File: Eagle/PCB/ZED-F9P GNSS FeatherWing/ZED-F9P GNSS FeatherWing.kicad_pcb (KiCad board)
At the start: 2 copper layers, 50.8 x 22.9 mm, 43 parts, among them CON1 MICROBUILDER_USBFCI_10103594_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, J1 Coupler_v2_Coupler_v2-rescue_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, Q1 DMG2305, U1 ZED-F9P_ZED-F9P, U2 SPX3819-3.3, X1 SMA-142-0711-821/826

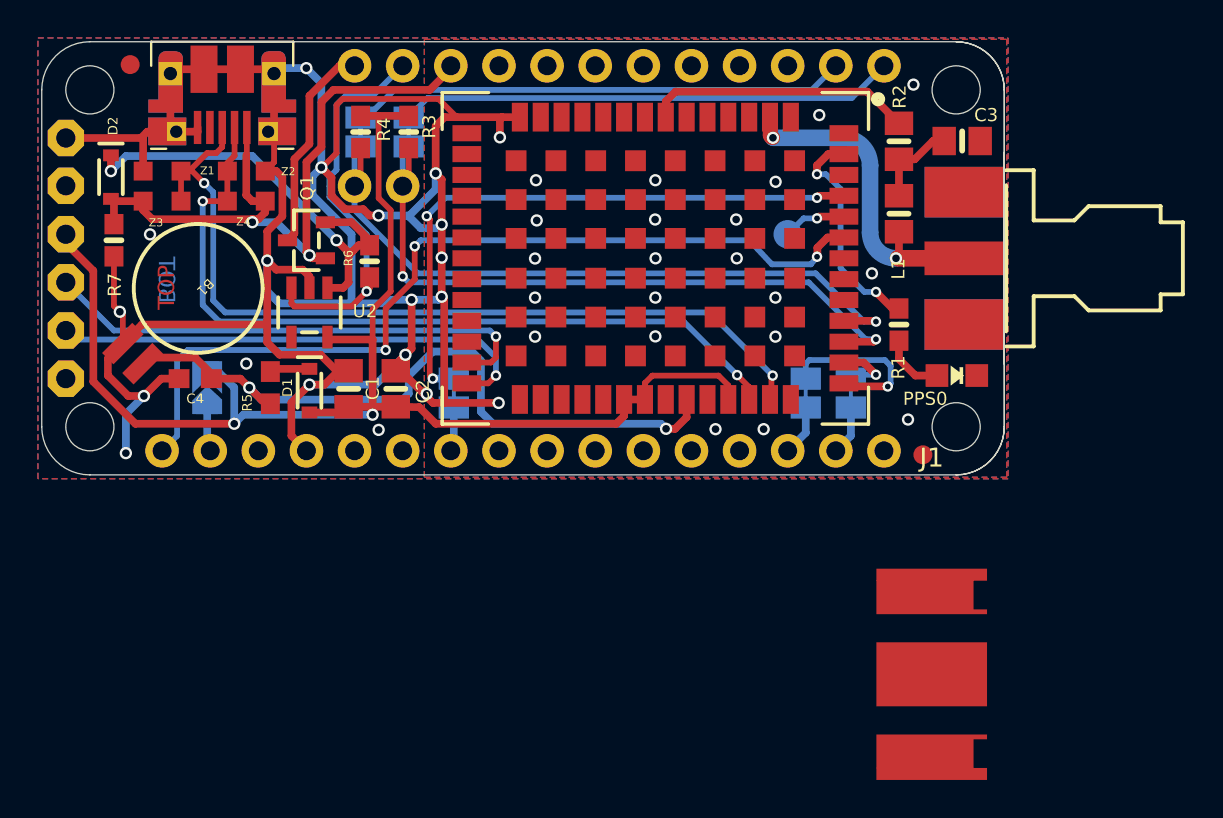
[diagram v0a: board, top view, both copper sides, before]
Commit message: V2 Release
Released to fab.
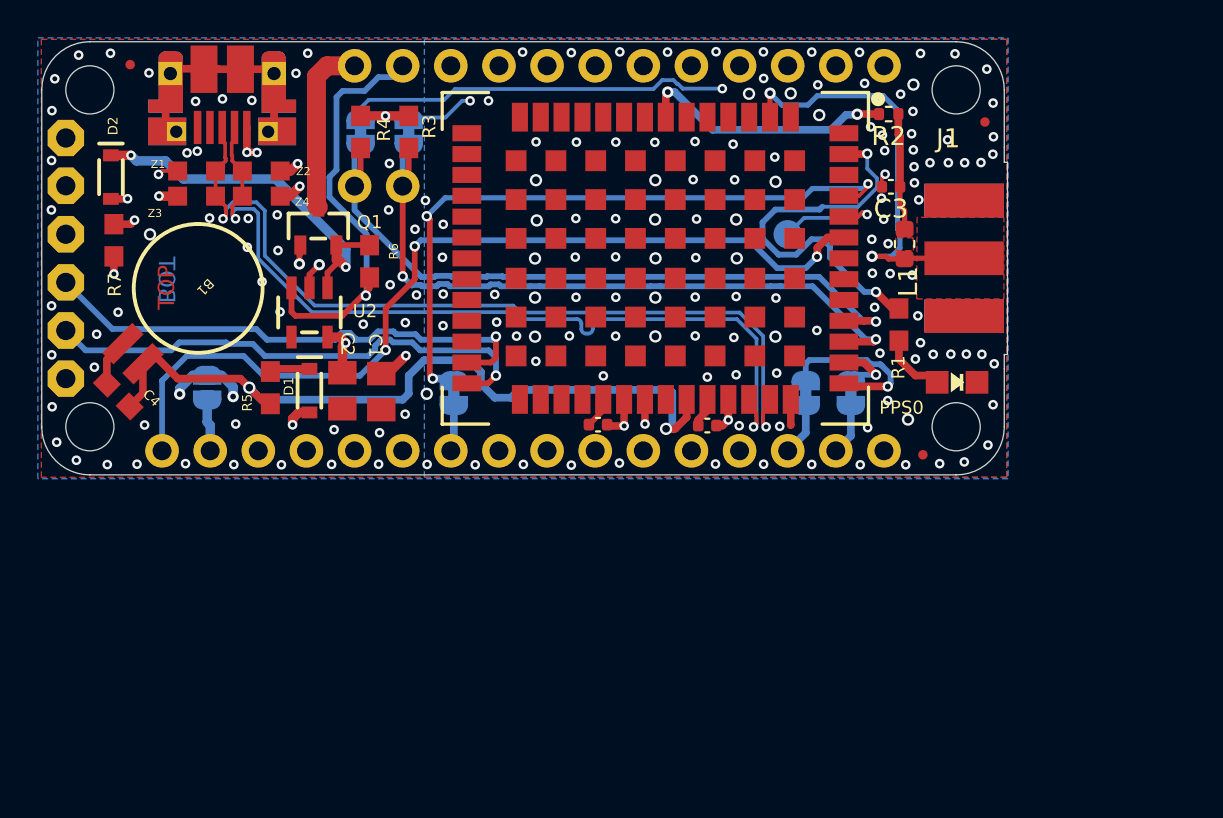
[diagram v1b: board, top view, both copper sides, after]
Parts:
- removed X1: SMA-142-0711-821/826, ZED-F9P GNSS FeatherWing:J502-ND-142-0711-821_826_133
- added C5: C_Small_US, Capacitor_SMD:C_0402_1005Metric, F.Cu at (158.2, 113.8)
- added C6: C_Small_US, Capacitor_SMD:C_0402_1005Metric, F.Cu at (152.5, 113.8)
- added FID3: FIDUCIAL"", Fiducial:Fiducial_0.5mm_Mask1mm, F.Cu at (172.9, 97.8)
- C3: value 10nF -> 47pF; footprint ZED-F9P GNSS FeatherWing:0805-NO -> Capacitor_SMD:C_0402_1005Metric
- FID1, FID2: footprint ZED-F9P GNSS FeatherWing:FIDUCIAL_1MM -> Fiducial:Fiducial_0.5mm_Mask1mm
- INT0, RX0, SCL0, SDA0, TX0: footprint ZED-F9P GNSS FeatherWing:SOLDERJUMPER_CLOSEDWIRE -> Jumper:SolderJumper-2_P1.3mm_Bridged_RoundedPad1.0x1.5mm
- J1: value Coupler_v2_Coupler_v2-rescue_SMA-Coupler_v1-rescue -> EdgeMount_SMA; footprint Coupler_v1:SMA_Molex_732511150_v3 -> Coupler_v1:SMA_Molex_0732512120
- L1: value 27nH -> 100nH; footprint ZED-F9P GNSS FeatherWing:0805-NO -> Inductor_SMD:L_0603_1608Metric
- R2: footprint ZED-F9P GNSS FeatherWing:0805-NO -> Resistor_SMD:R_0402_1005Metric
- R6, R7: value 100K -> 10K
- U1: value ZED-F9P_ZED-F9P -> ZED-F9P-15B
- UNK3.3V0: footprint ZED-F9P GNSS FeatherWing:SOLDERJUMPER_ARROW_NOPASTE -> Jumper:SolderJumper-2_P1.3mm_Open_RoundedPad1.0x1.5mm
- moved J1 22.0 mm to (171.8, 105.0)
- moved C3 4.47 mm to (167.9, 101.2), turned to 180 degrees
- moved C4 4.15 mm to (127.1, 112.2), turned to 135 degrees
- moved C2 2.82 mm to (139.0, 112.0), turned to -90 degrees
- moved Z3 1.84 mm to (131.3, 101.7)
- moved Z1 1.82 mm to (131.3, 100.4)
- moved C1 1.73 mm to (141.0, 112.0), turned to -90 degrees
- moved L1 1.63 mm to (168.6, 104.2)
- moved R2 1.54 mm to (167.8, 97.4), turned to 180 degrees
- moved Q1 0.98 mm to (137.7, 103.3), turned to 0 degrees
- moved Z4 0.84 mm to (134.7, 101.7)
- moved Z2 0.79 mm to (134.7, 100.4)
- moved PPS0 0.36 mm to (171.4, 111.5)
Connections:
- J1 pad 1: unconnected-(J1-Signal-Pad1) -> /ANT
- J1 pad 2: unconnected-(J1-GND-Pad2) -> GND
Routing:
- net GND: track 156.3 -> 24.6 mm, vias 41 -> 180
- net 3.3V: track 75.0 -> 17.9 mm, vias 2 -> 9
- net VBUS: track 36.5 -> 7.16 mm, vias 2 -> 7
- net /TP: track 11.8 -> 20.7 mm
- net Net-(MS1-GPIOSDA): track 26.4 -> 31.6 mm, vias 0 -> 1
- net /ANT: track 17.8 -> 22.7 mm
- net Net-(MS1-GPIOSCL): track 26.2 -> 30.8 mm, vias 0 -> 1
- net /EXTINT: track 32.3 -> 35.4 mm
- net /D-: track 42.1 -> 45.2 mm
- net /VBACKUP: track 37.4 -> 40.4 mm
- net /SAFEBOOT: track 3.35 -> 6.09 mm
- net Net-(Q1-S): track 22.9 -> 20.3 mm
- net VBAT: track 11.1 -> 9.18 mm
- net Net-(L1-P$1): track 4.71 -> 6.22 mm
- net /EN: track 21.1 -> 22.4 mm
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- added copper zone on In1.Cu, net 3.3V
- added copper zone on In1.Cu, net GND
- added copper zone on In2.Cu, net GND
- added copper zone on In1.Cu, net VBUS
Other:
- copper layers 2 -> 4
- board text added: "github.com/laberge1/ZED-F9P_FeatherWing_USB"
- board text removed: "3V3"
- board text removed: "FeatherWing"
